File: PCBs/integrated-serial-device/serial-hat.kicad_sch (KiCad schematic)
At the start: 22 parts, among them CN1 Modem port, CN2 Modem out 3, CN3 Printer port, J1 Rpi headers, J3 Conn_01x02_Pin, K1 Quicktake, K2 ImageWriter, SW1 Modem To Proxy, SW2 Modem to Quicktake, SW3 Modem out 3, SW5 Printer to Proxy, SW6 Printer to ImageWriter, SW7 SW_SPST, SW8 SW_Slide_DPDT SHOU HAN MSK-22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, U1 MAX3232, U2 PC817C-S

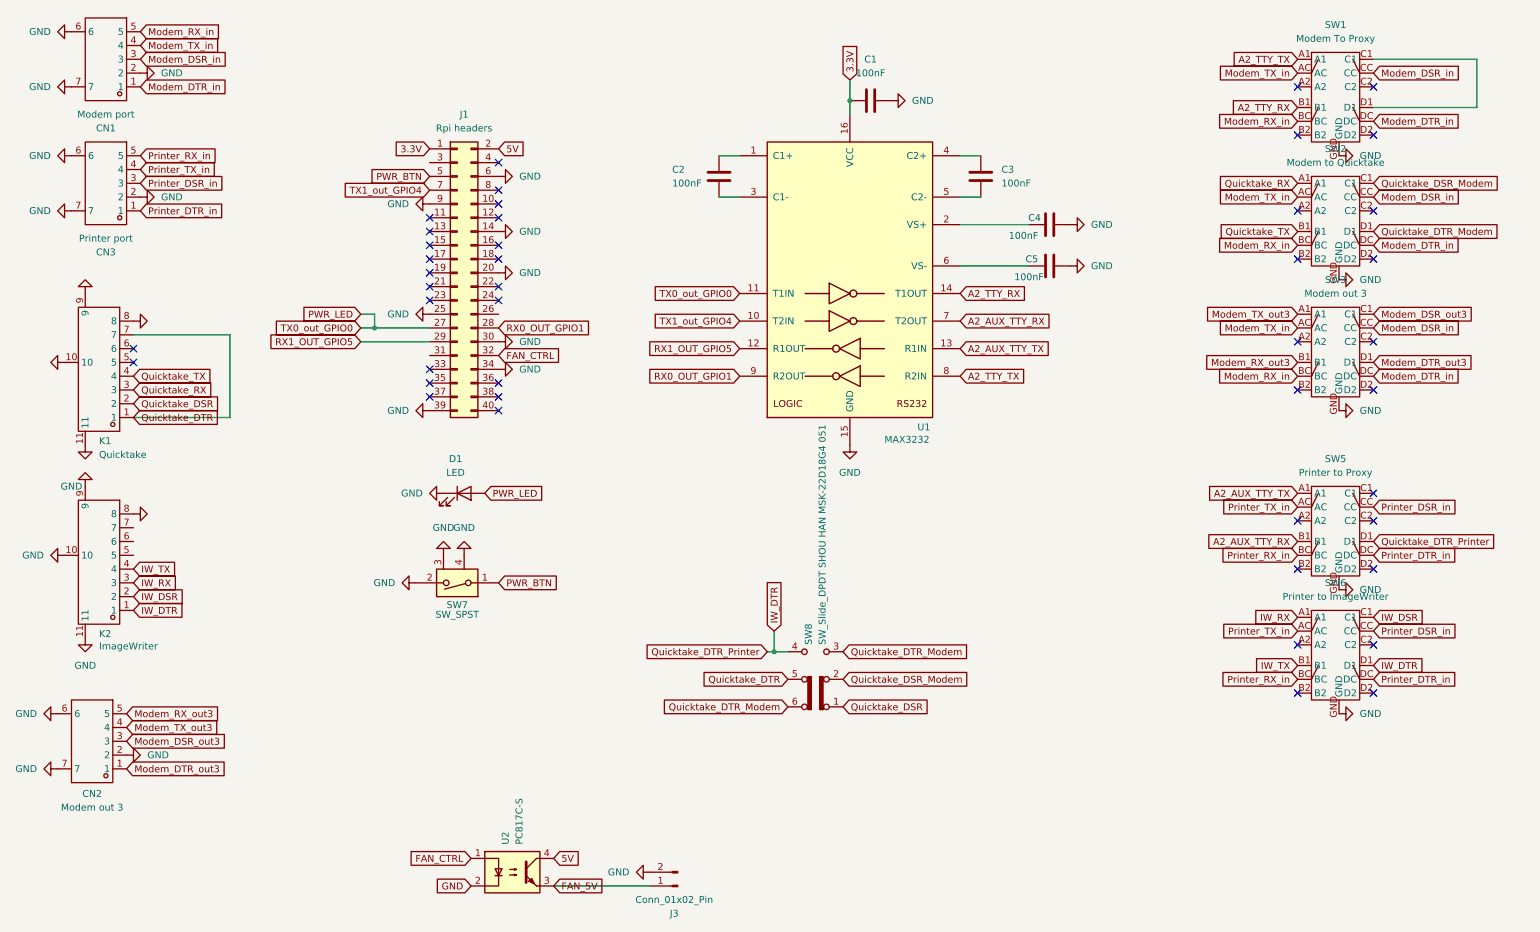
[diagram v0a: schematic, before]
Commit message: Update to new lib
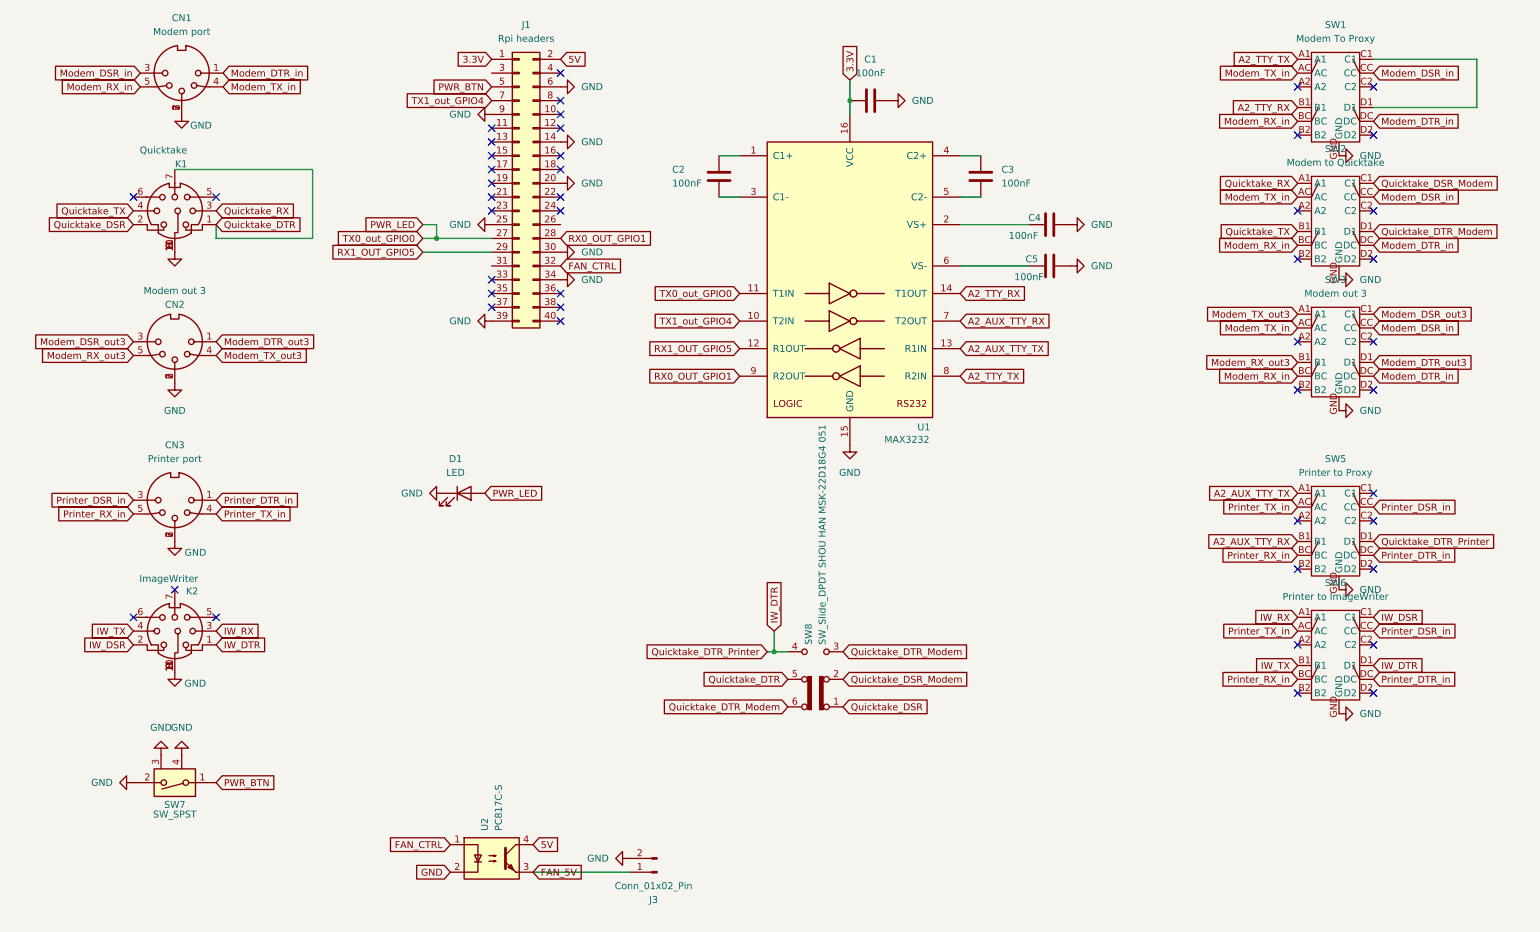
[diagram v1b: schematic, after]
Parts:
- CN1, CN2, CN3: footprint DIN5:CONN-TH_DIN-504-M10 -> Colins-Kicad:DIN-5-M C23689428; symbol DIN:DIN-504 -> Colins-Kicad:DIN-5_180degree
- K1, K2: footprint DIN5:MINI-DIN8 -> Colins-Kicad:MINI-DIN8-F C20611694; symbol DIN:DIN-802 -> Colins-Kicad:Serial_Mini-DIN-8
- SW1, SW2, SW3, SW5, SW6: footprint DIN5:4PDT piano switch -> Colins-Kicad:4PDT 12 pins Piano Switch; symbol DIN:4PDT_switch -> Colins-Kicad:4PDT_switch
- SW7: footprint DIN5:SPST_power_switch -> Colins-Kicad:SPST momentary switch C6575016
- SW8: footprint DIN5:DPDT slide switch C7507433 -> Colins-Kicad:DPDT slide switch C7507433
- U2: footprint Package_SO:SOP-4_3.8x4.1mm_P2.54mm -> Colins-Kicad:PC817C-S C3008369
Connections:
- no-connect marks 44 -> 47
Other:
- moved on the sheet: J1, J3, SW7, U2
